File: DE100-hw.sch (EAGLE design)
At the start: 50 parts, among them IC3 74HC14D, IC4 74HC14D, U1 TLP521-4(GB), U2 TLP521-4(GB), X1 22-23-2041, X2 22-23-2031, X3 22-23-2101

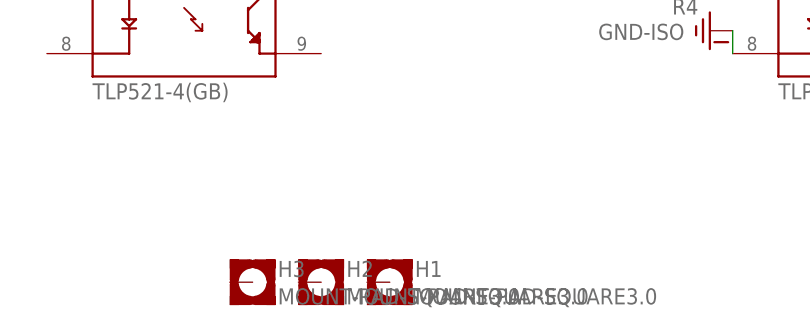
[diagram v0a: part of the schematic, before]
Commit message: change route
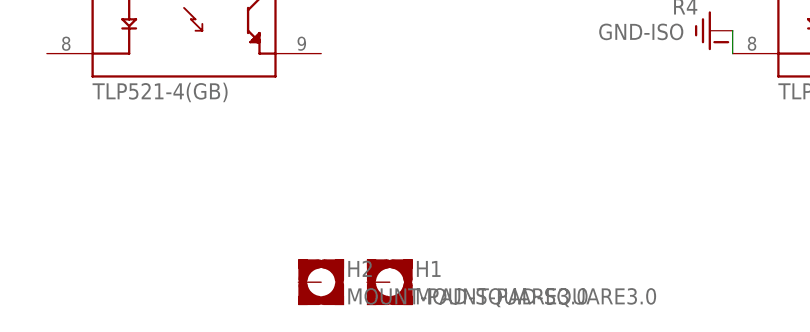
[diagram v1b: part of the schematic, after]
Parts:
- removed H3: MOUNT-PAD-SQUARE3.0, holes:MOUNT-PAD-SQUARE3.0
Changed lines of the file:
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@@
 <part name="H1" library="holes" library_urn="urn:adsk.eagle:library:237" deviceset="MOUNT-PAD-SQUARE" device="3.0" package3d_urn="urn:adsk.eagle:package:14290/1"/>
 <part name="H2" library="holes" library_urn="urn:adsk.eagle:library:237" deviceset="MOUNT-PAD-SQUARE" device="3.0" package3d_urn="urn:adsk.eagle:package:14290/1"/>
-<part name="H3" library="holes" library_urn="urn:adsk.eagle:library:237" deviceset="MOUNT-PAD-SQUARE" device="3.0" package3d_urn="urn:adsk.eagle:package:14290/1"/>
 </parts>
 <sheets>
@@
 <attribute name="VALUE" x="165.354" y="2.6162" size="1.778" layer="96"/>
 </instance>
-<instance part="H3" gate="G$1" x="154.94" y="5.08" smashed="yes">
-<attribute name="NAME" x="157.734" y="5.6642" size="1.778" layer="95"/>
-<attribute name="VALUE" x="157.734" y="2.6162" size="1.778" layer="96"/>
-</instance>
 </instances>
